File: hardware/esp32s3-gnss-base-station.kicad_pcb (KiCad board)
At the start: 4 copper layers, 108 x 108 mm, 64 parts, among them CN1 JST 2mm, J1 PWR_BYPASS, J2 OLED, Q1 MMDT3904, SW1 SS-12D10L5, U1 ESP32-S3-WROOM-1-N16R8, U2 ZED-F9P-04B, U3 CP2102-GMR, U4 TP4054, U5 SY8089AAAC, U6 BWMCX-KE

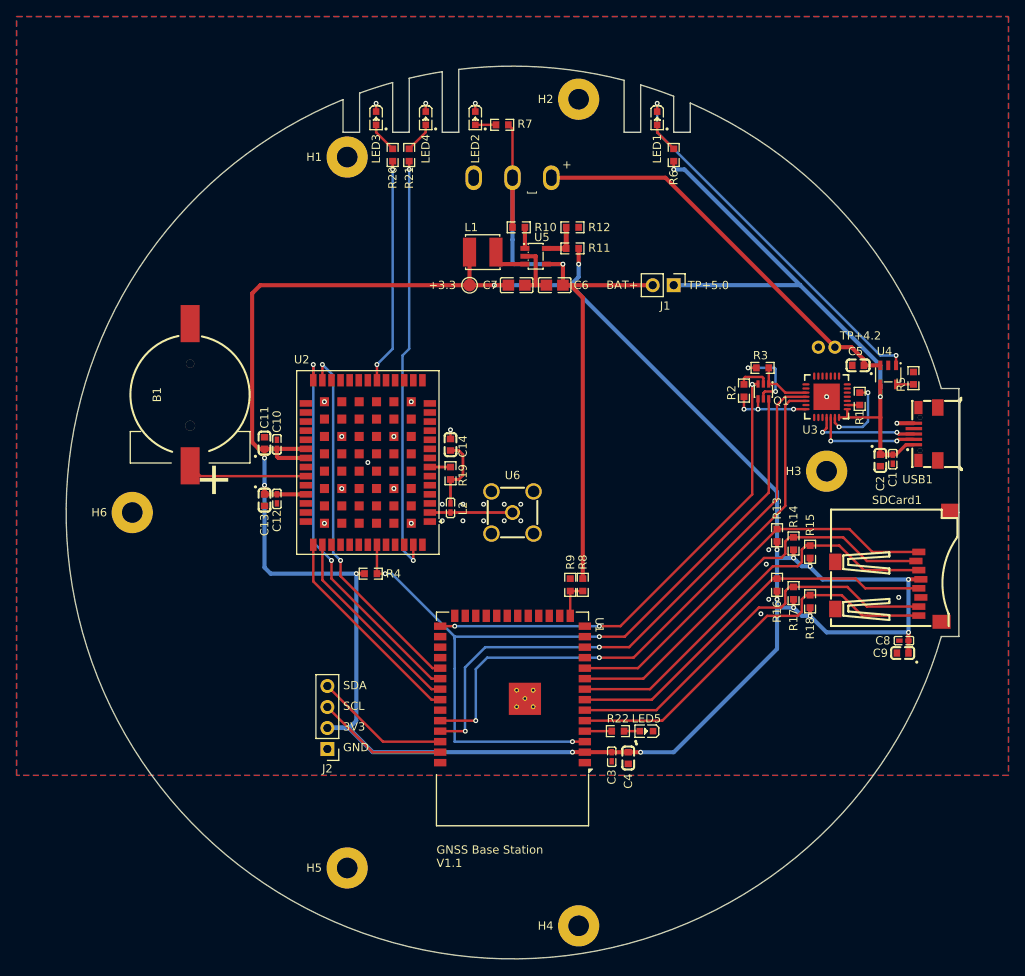
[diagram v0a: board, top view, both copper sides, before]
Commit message: Update PCB and export some images
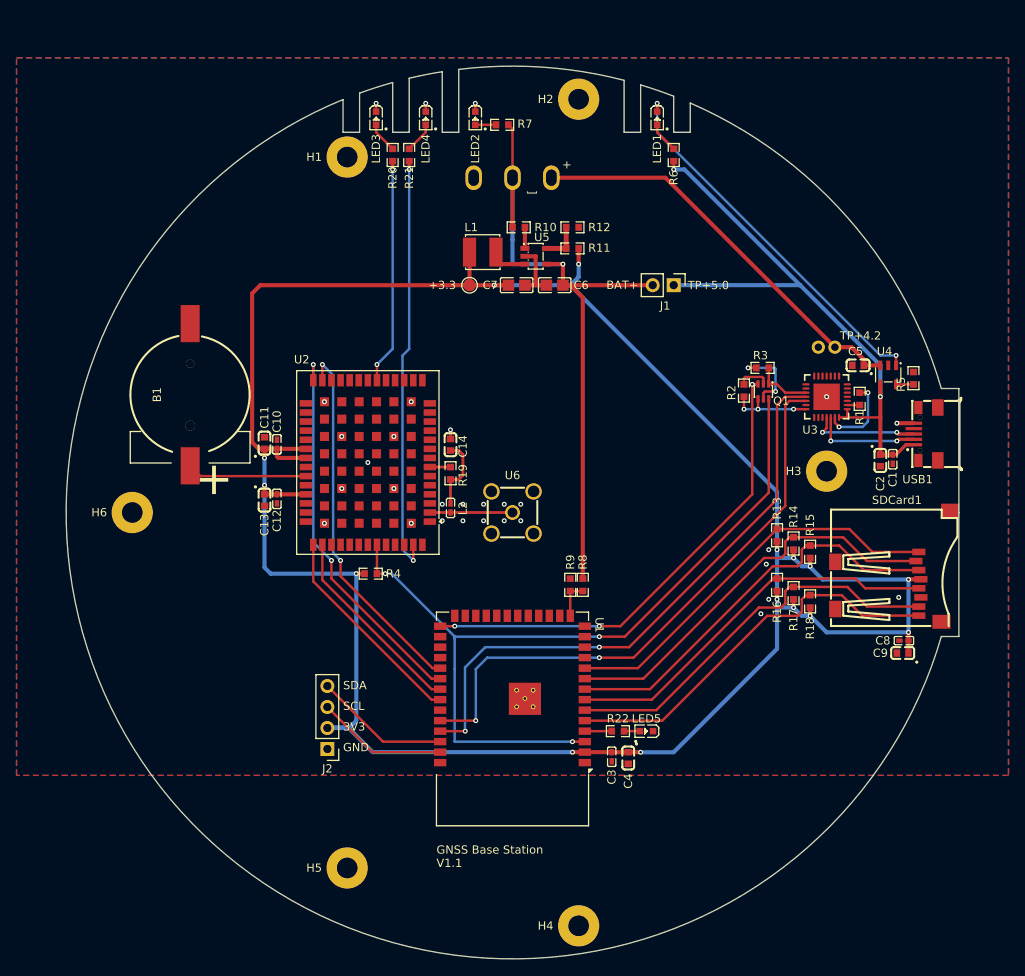
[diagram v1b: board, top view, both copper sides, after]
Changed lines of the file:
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@@
 			(crossoutdnponfab yes)
 			(subtractmaskfromsilk no)
-			(outputformat 1)
+			(outputformat 5)
 			(mirror no)
-			(drillshape 1)
+			(drillshape 0)
 			(scaleselection 1)
 			(outputdirectory "")
@@
 		)
 		(embedded_fonts no)
-		(model "${KICAD9_3DMODEL_DIR}/RF_GPS.3dshapes/ublox_ZED.step"
+		(model "${KIPRJMOD}/libs/LCSC.3dshapes/LCC-LGA-102_L22.0-W17.0_FM660.wrl"
 			(offset
 				(xyz 0 0 0)
@@
 			)
 			(rotate
-				(xyz 0 0 0)
+				(xyz -0 -0 90)
 			)
 		)
@@
 	)
 	(footprint "LCSC:TF-SMD_TF-001B"
+		(locked yes)
 		(layer "F.Cu")
 		(at 146 106.5 180)
@@
 		(polygon
 			(pts
-				(xy 40 40) (xy 160 40) (xy 160 131.8) (xy 40 131.8)
+				(xy 40 45) (xy 160 45) (xy 160 131.8) (xy 40 131.8)
 			)
 		)
